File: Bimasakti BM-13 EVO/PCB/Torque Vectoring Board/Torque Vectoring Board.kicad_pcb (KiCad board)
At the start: 2 copper layers, 108 x 104.9 mm, 34 parts, among them J1 SIGNAL 1, J2 SIGNAL 2, J3 wsout1, J4 wsout2, U3 SN65HVD230, U4 SN65HVD230, U5 ADS1115IDGS

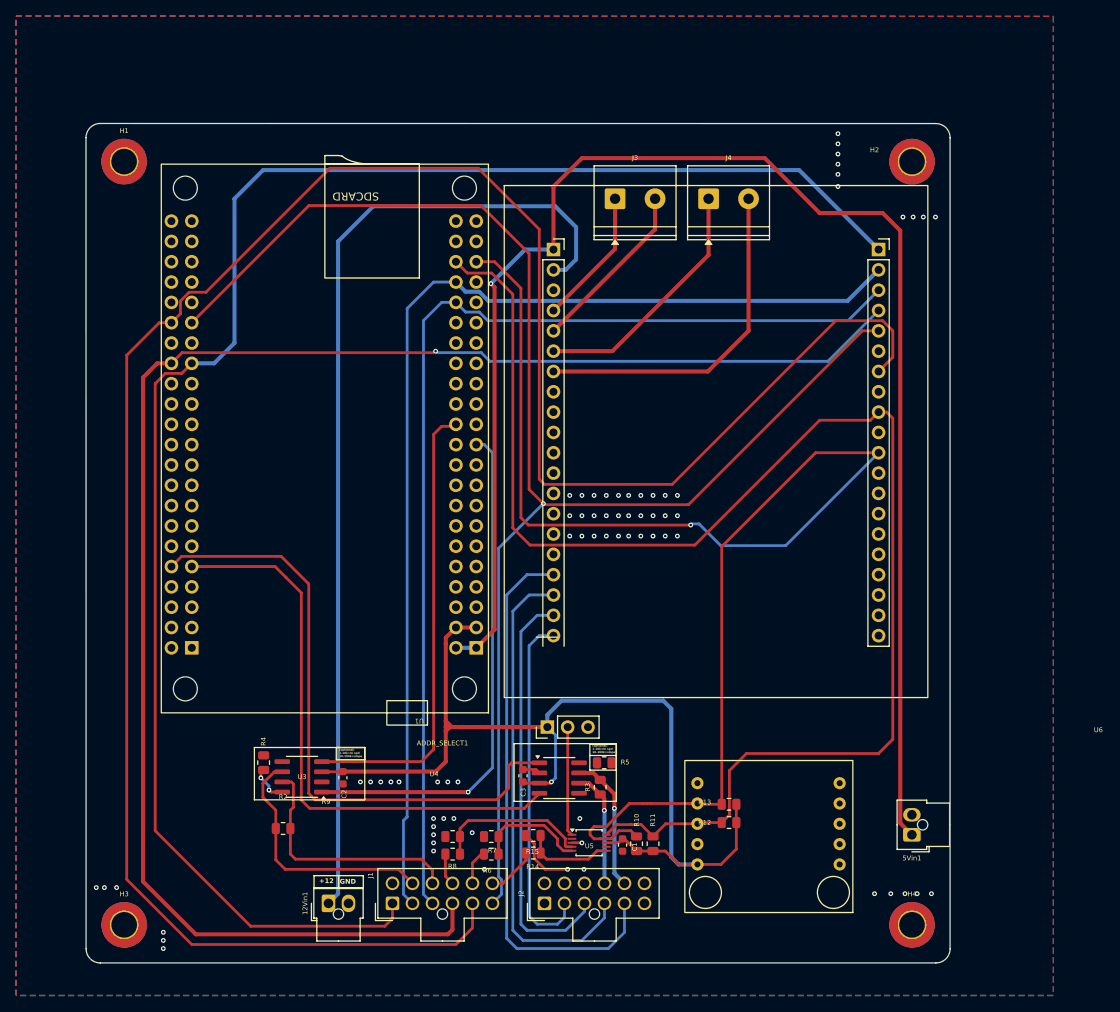
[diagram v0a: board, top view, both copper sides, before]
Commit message: tv dengan pdm kecil
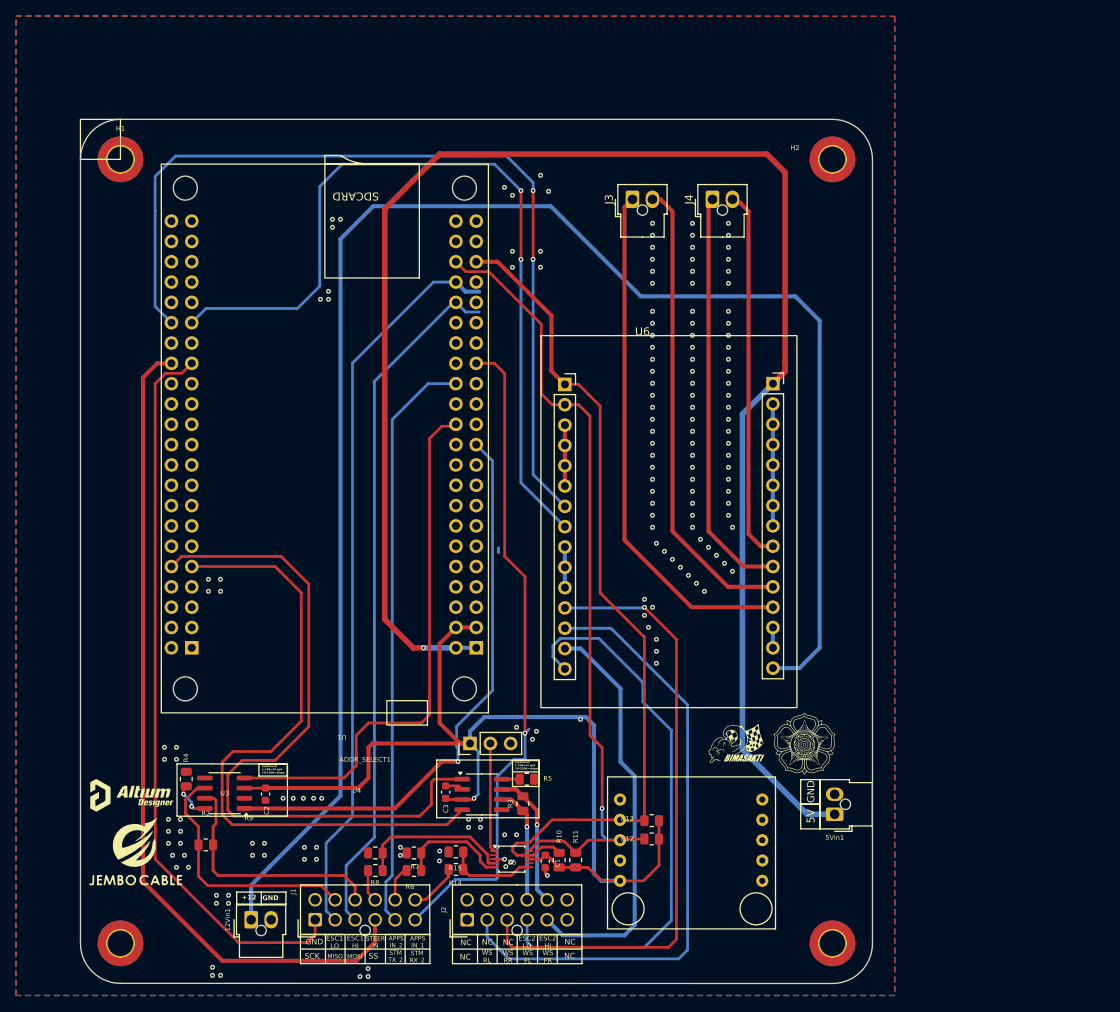
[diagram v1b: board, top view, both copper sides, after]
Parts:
- added G***: LOGO, 0_logo:altium 12x12, F.Cu at (50.5, 117.5)
- added G***: LOGO, 0_logo:logo bimsak, F.Cu at (126.0, 111.0)
- added G***: LOGO, 0_logo:ugm 7.8x7.8, F.Cu at (134.5, 111.0)
- added a: LOGO, 0_logo:11jembo_tulisan_12x8.7, F.Cu at (51.0, 124.5)
- J3, J4: footprint TerminalBlock_Phoenix:TerminalBlock_Phoenix_PT-1,5-2-5.0-H_1x02_P5.00mm_Horizontal -> Connector_Molex:Molex_Nano-Fit_105309-xx02_1x02_P2.50mm_Vertical
- U6: footprint 0_CUSTOM_PCB:wheelspeed -> 0_WHEELSPEED:Untitled
- moved U6 25.6 mm to (114.3, 60.0)
- moved H4 10.2 mm to (138.0, 136.0)
- moved 5Vin1 9.99 mm to (138.3, 119.9)
- moved H2 9.95 mm to (138.0, 38.0)
- moved 12Vin1 9.88 mm to (65.3, 133.0)
- moved C1 9.88 mm to (102.1, 125.8)
- moved J1 9.88 mm to (73.3, 133.0)
- moved J2 9.88 mm to (92.3, 133.0)
- moved R10 9.88 mm to (103.8, 125.6)
- moved R12 9.88 mm to (115.4, 123.0)
- moved R13 9.88 mm to (115.4, 120.7)
- moved R4 9.88 mm to (57.2, 115.5)
- moved R5 9.88 mm to (99.8, 115.5)
- moved R8 9.88 mm to (80.9, 126.9)
- moved U5 9.88 mm to (97.9, 125.5)
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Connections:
- J1 pad 5: STM_TX -> STM_TX_2
- J1 pad 6: STM_RX -> STM_RX_2
- J2 pad 1: unconnected-(J2-Pin_1-Pad1) -> GND
- J2 pad 12: unconnected-(J2-Pin_12-Pad12) -> GND
- J2 pad 6: unconnected-(J2-Pin_6-Pad6) -> GND
- J2 pad 7: unconnected-(J2-Pin_7-Pad7) -> GND
- J2 pad 8: unconnected-(J2-Pin_8-Pad8) -> GND
- J2 pad 9: unconnected-(J2-Pin_9-Pad9) -> GND
- U1 pad 28: unconnected-(U1-PC12-Pad28) -> STM_TX_2
- U1 pad 29: unconnected-(U1-PD2-Pad29) -> STM_RX_2
- U6 pad 10: GND -> WS_RRo
- U6 pad 11: GND -> WS_FLo
- U6 pad 12: GND -> WS_FRo
- U6 pad 13: GND -> SDA
- U6 pad 14: GND -> SCL
- U6 pad 3: GND -> STM_TX
- U6 pad 4: WS_FRo -> STM_RX
- U6 pad 5: WS_FLo -> WS_RR
- U6 pad 6: WS_RRo -> WS_RL
- U6 pad 7: WS_RLo -> WS_FR
- U6 pad 8: GND -> WS_FL
- U6 pad 9: GND -> WS_RLo
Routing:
- net STM_TX: track 271.9 -> 110.9 mm, vias 0 -> 2
- net SCK: track 208.9 -> 91.7 mm
- net SS: track 204.4 -> 104.2 mm, vias 1 -> 0
- net STM_RX_2: track 0.00 -> 84.7 mm, vias 0 -> 1
- net STM_RX: track 186.6 -> 102.3 mm, vias 1 -> 2
- net 12V: track 123.3 -> 205.2 mm
- net SCL: track 178.7 -> 101.4 mm, vias 0 -> 1
- net STM_TX_2: track 0.00 -> 73.1 mm
- net SDA: track 168.4 -> 106.2 mm, vias 1 -> 0
- net WS_FRo: track 17.2 -> 65.0 mm
- net MOSI: track 133.7 -> 86.9 mm
- net MISO: track 137.9 -> 91.9 mm
- net WS_FLo: track 21.8 -> 58.6 mm
- net WS_RL: track 44.3 -> 78.8 mm
- net WS_RR: track 51.7 -> 77.8 mm, vias 0 -> 1
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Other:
- board size 108 x 104.9 mm -> 99 x 108 mm
- board text added: "5V"
- board text added: "APPS IN_1"
- board text added: "APPS IN_2"
- board text added: "ESC1 HI"
- board text added: "ESC1 LO"
- board text added: "ESC2 HI"
- board text added: "ESC2 LO"
- board text added: "MISO"
- board text added: "MOSI"
- board text added: "NC"
- board text added: "SCK"
- board text added: "SS"
- board text added: "STEER IN"
- board text added: "STM RX_2"
- board text added: "STM TX_2"
- board text added: "WS FL"
- board text added: "WS FR"
- board text added: "WS RL"
- board text added: "WS RR"
